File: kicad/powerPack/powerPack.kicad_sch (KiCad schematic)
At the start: 4 parts, among them U1 BQ24075RGT, U2 MT3608, U3 MT3608, U4 BQ27441DRZR-G1A

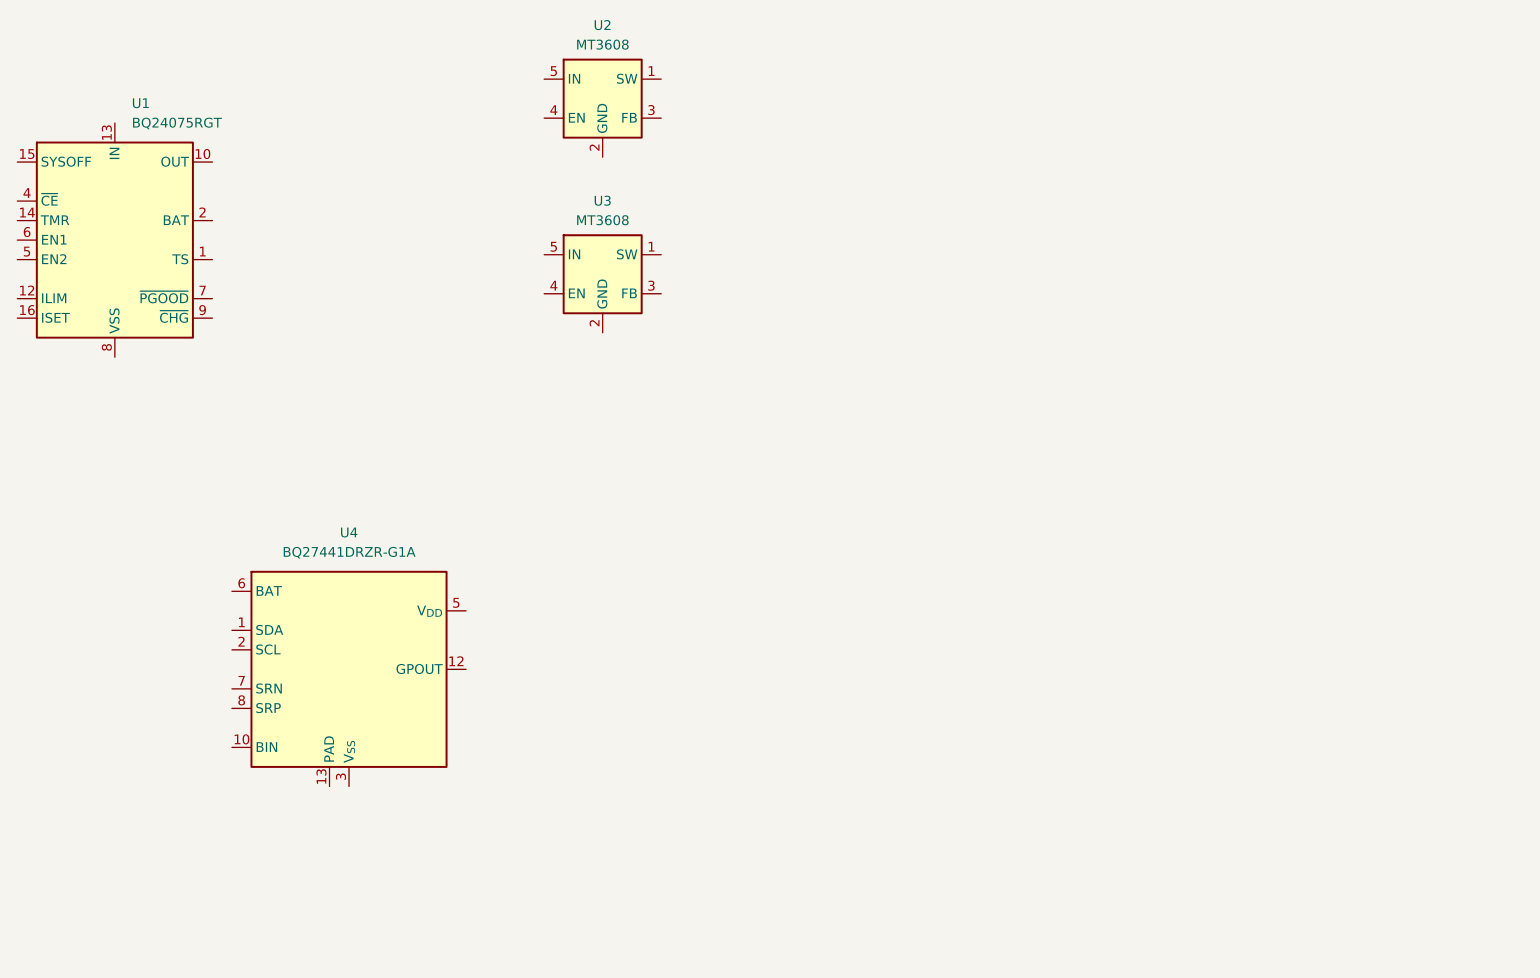
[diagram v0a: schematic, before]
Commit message: .
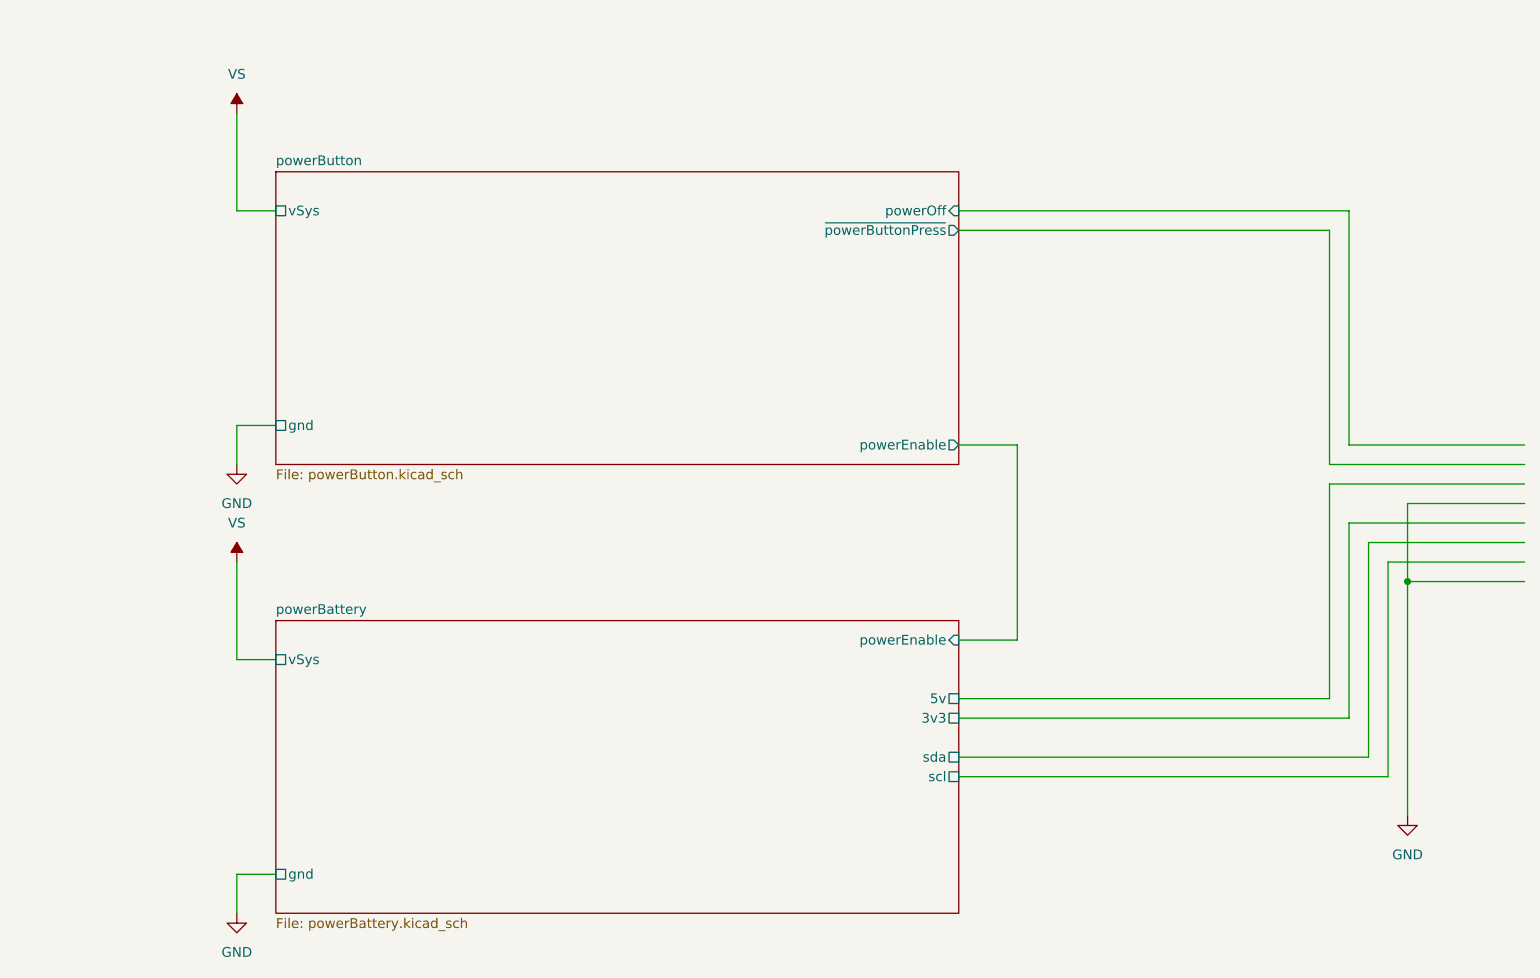
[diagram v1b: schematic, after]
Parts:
- removed U1: BQ24075RGT, Package_DFN_QFN:VQFN-16-1EP_3x3mm_P0.5mm_EP1.6x1.6mm, symbol Battery_Management:BQ24075RGT
- removed U2, U3: MT3608, Package_TO_SOT_SMD:SOT-23-6, symbol Regulator_Switching:MT3608
- removed U4: BQ27441DRZR-G1A, Package_SON:Texas_S-PDSO-N12, symbol Battery_Management:BQ27441DRZR-G1A
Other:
- added sheet powerBattery (powerBattery.kicad_sch)
- added sheet powerButton (powerButton.kicad_sch)
